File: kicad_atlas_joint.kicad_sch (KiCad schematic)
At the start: 24 parts, among them IC1 AS5600, J1 Screw_Terminal_01x07, J3 Screw_Terminal_01x06, SW1 SW_Push, U1 STM32F411CEUx, U2 INA226, U3 LM2596S-3.3

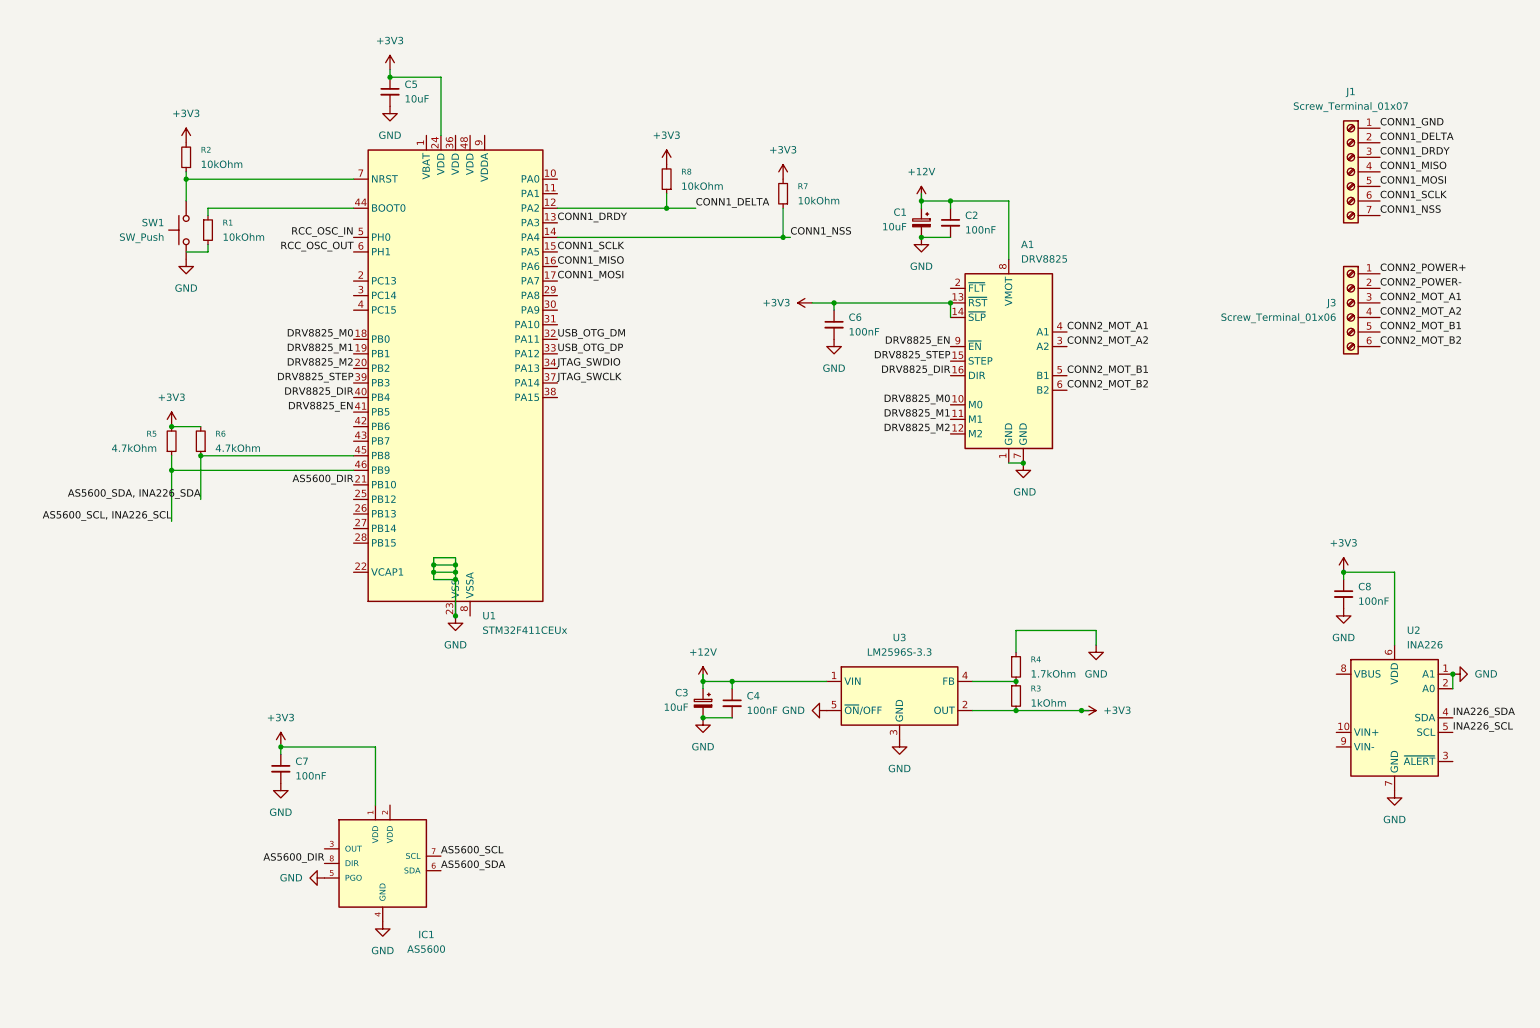
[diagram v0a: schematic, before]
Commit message: changes
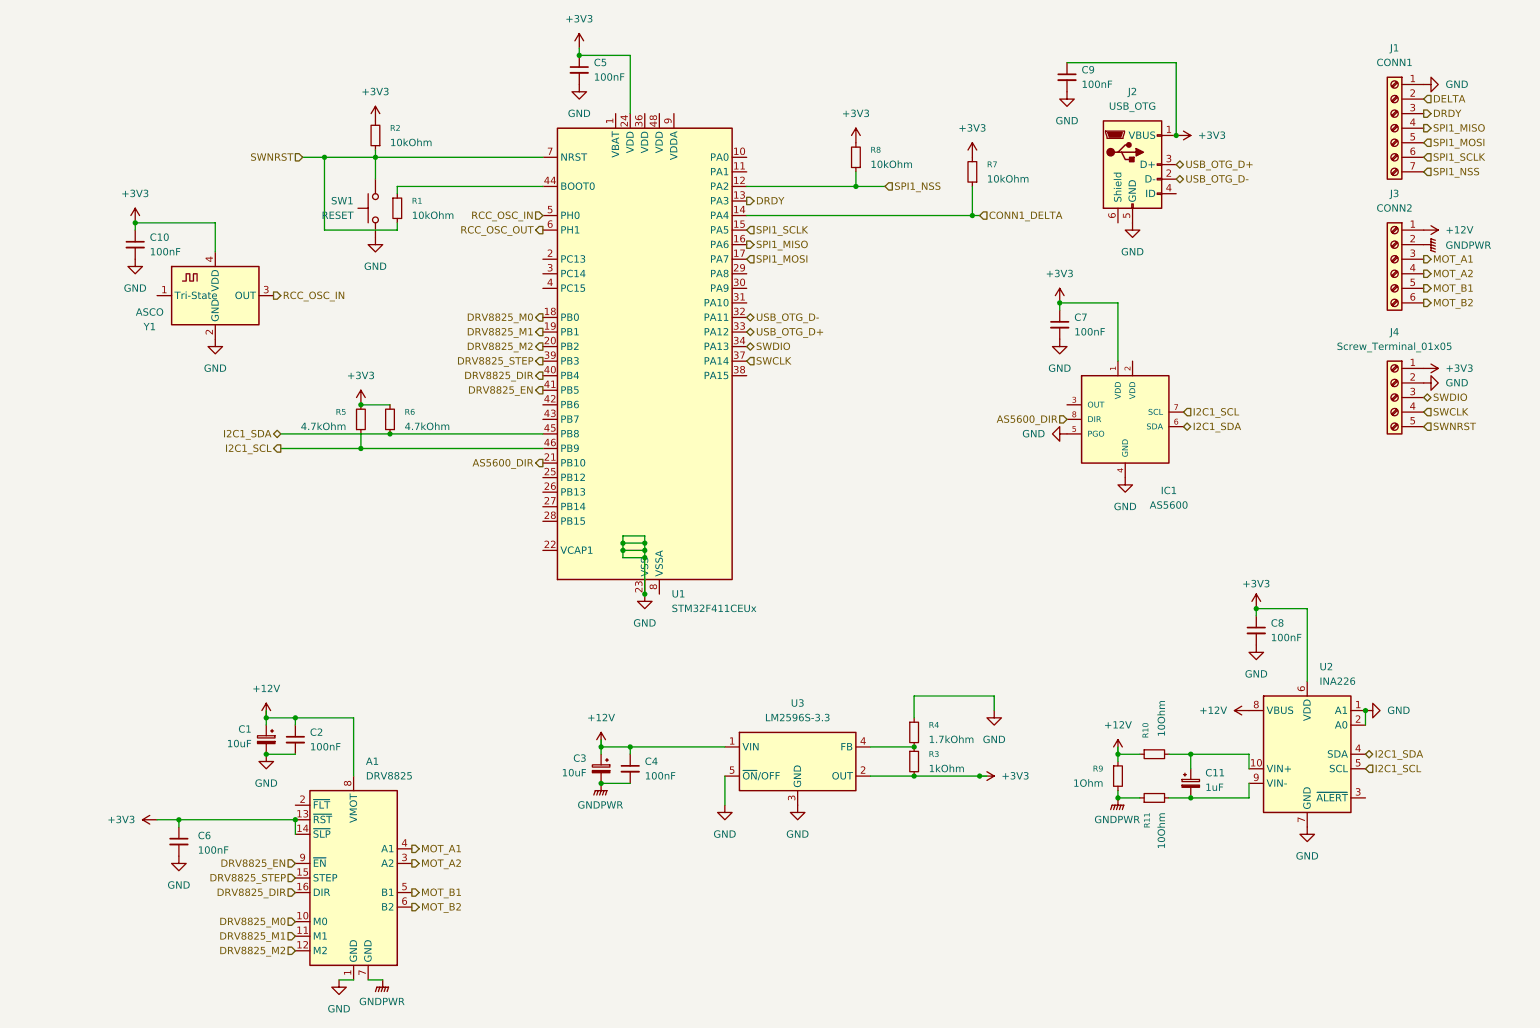
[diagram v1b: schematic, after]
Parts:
- added C10, C9: 100nF, symbol Device:C_Small
- added C11: 1uF, symbol Device:C_Polarized_Small
- added J2: USB_OTG, symbol Connector:USB_OTG
- added J4: Screw_Terminal_01x05, symbol Connector:Screw_Terminal_01x05
- added R10, R11: 10Ohm, symbol Device:R_Small
- added R9: 1Ohm, symbol Device:R_Small
- added Y1: ASCO, Oscillator:Oscillator_SMD_Abracon_ASCO-4Pin_1.6x1.2mm, symbol Oscillator:ASCO
- C5: value 10uF -> 100nF
- J1: value Screw_Terminal_01x07 -> CONN1
- J3: value Screw_Terminal_01x06 -> CONN2
- SW1: value SW_Push -> RESET
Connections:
- net AS5600_SCL, INA226_SCL is gone; now on net I2C1_SCL: R5.1, U1.46 (PB9)
- net AS5600_SDA, INA226_SDA is gone; now on net I2C1_SDA: R6.1, U1.45 (PB8)
- net CONN1_GND is gone; now on net GND: J1.1 (Pin_1)
- net CONN2_POWER+ is gone; now on net +12V: J3.1 (Pin_1)
- net INA226_SCL is gone; now on net I2C1_SCL: U2.5 (SCL)
- net INA226_SDA is gone; now on net I2C1_SDA: U2.4 (SDA)
- net +12V: now also U2.8 (VBUS), R10.1, R9.1
- net +3V3: now also C10.1, C9.1, J2.1 (VBUS), J4.1 (Pin_1), Y1.4 (VDD)
- net CONN1_DELTA: now also R7.1, U1.14 (PA4); no longer J1.2 (Pin_2), R8.1, U1.12 (PA2)
- net GND: now also C10.2, C9.2, J2.5 (GND), J4.2 (Pin_2), Y1.2 (GND); no longer A1.7 (GND), C3.2, C4.2
- net RCC_OSC_IN: now also Y1.3 (OUT)
- net SWNRST: now reaches R2.1, SW1.1, U1.7 (NRST)
- net SWNRST: now also R1.2, J4.5 (Pin_5)
- net at U2.10 (VIN+): now also C11.1, R10.2
- net at U2.9 (VIN-): now also C11.2, R11.2
- net AS5600_SCL renamed I2C1_SCL
- net AS5600_SDA renamed I2C1_SDA
- net CONN1_DRDY renamed DRDY
- net CONN1_MISO renamed SPI1_MISO
- net CONN1_MOSI renamed SPI1_MOSI
- removed net CONN1_NSS: J1.7 (Pin_7), R7.1, U1.14 (PA4)
- net CONN1_SCLK renamed SPI1_SCLK
- net CONN2_MOT_A1 renamed MOT_A1
- net CONN2_MOT_A2 renamed MOT_A2
- net CONN2_MOT_B1 renamed MOT_B1
- net CONN2_MOT_B2 renamed MOT_B2
- net CONN2_POWER- renamed GNDPWR
- net GNDPWR: now also A1.7 (GND), C3.2, C4.2, R11.1, R9.2
- net JTAG_SWCLK renamed SWCLK
- net SWCLK: now also J4.4 (Pin_4)
- net JTAG_SWDIO renamed SWDIO
- net SWDIO: now also J4.3 (Pin_3)
- net USB_OTG_DM renamed USB_OTG_D-
- net USB_OTG_D-: now also J2.2 (D-)
- net USB_OTG_DP renamed USB_OTG_D+
- net USB_OTG_D+: now also J2.3 (D+)
- new net DELTA: J1.2 (Pin_2)
- new net SPI1_NSS: J1.7 (Pin_7), R8.1, U1.12 (PA2)
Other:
- moved on the sheet: A1, C1, C2, C3, C4, C5, C6, C7, C8, IC1, J1, J3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
